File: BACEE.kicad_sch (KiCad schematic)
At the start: 13 parts, among them U1 24LC1025, U2 ATMEGA328-AU, U3 DS1337_PD, Y1 Crystal, Y2 Crystal

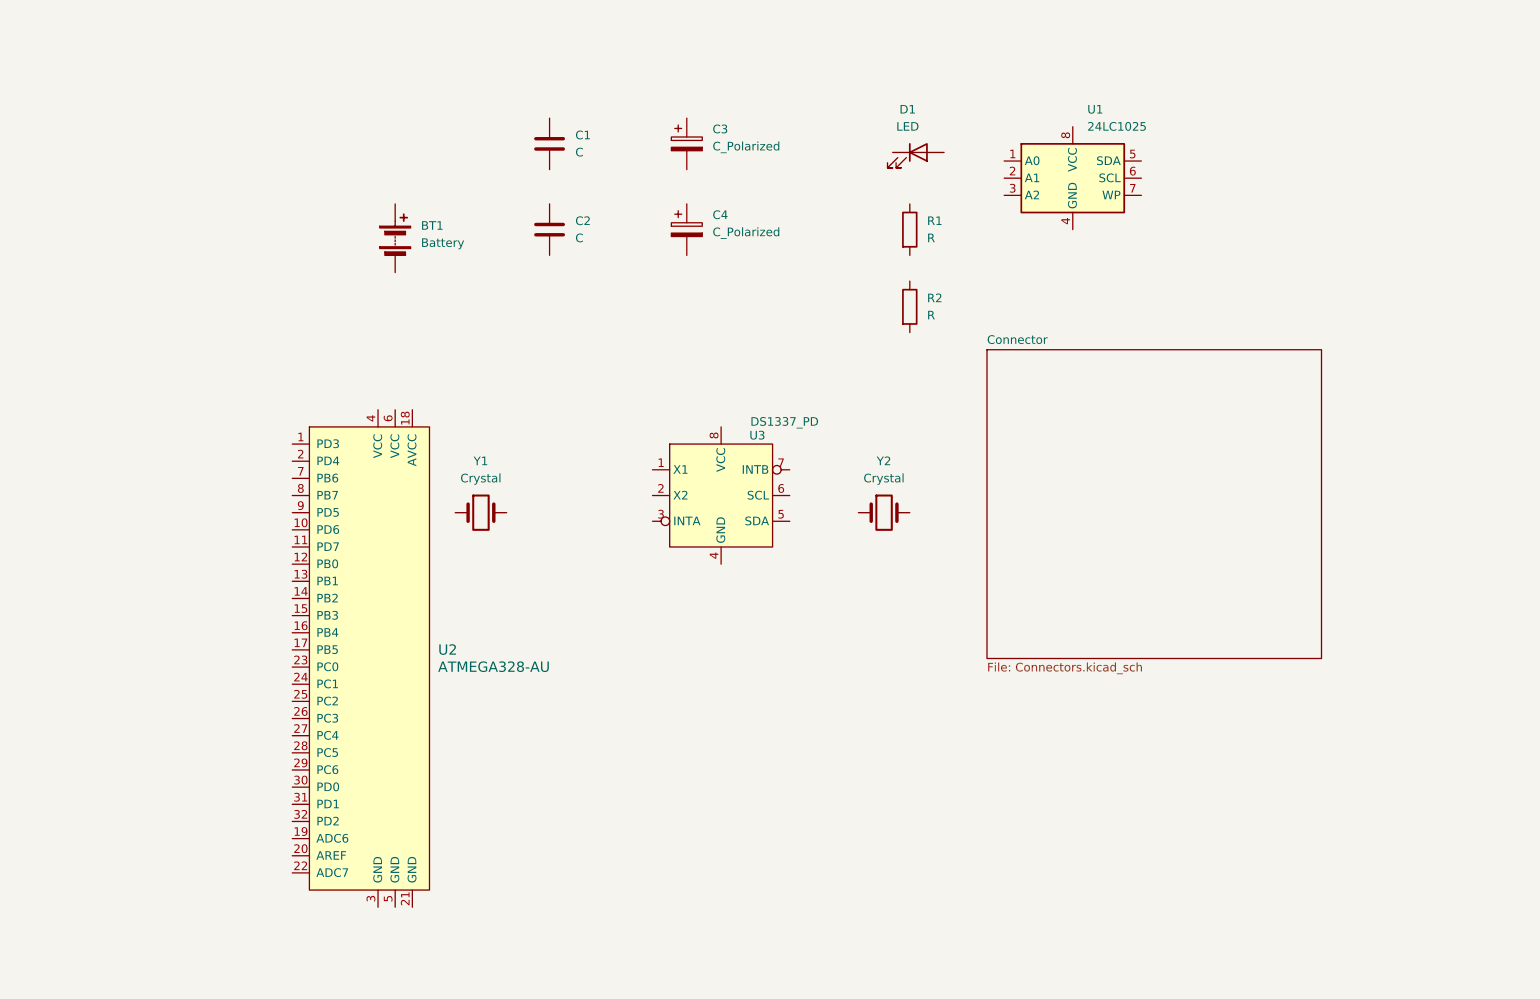
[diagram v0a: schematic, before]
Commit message: Arranged symbols
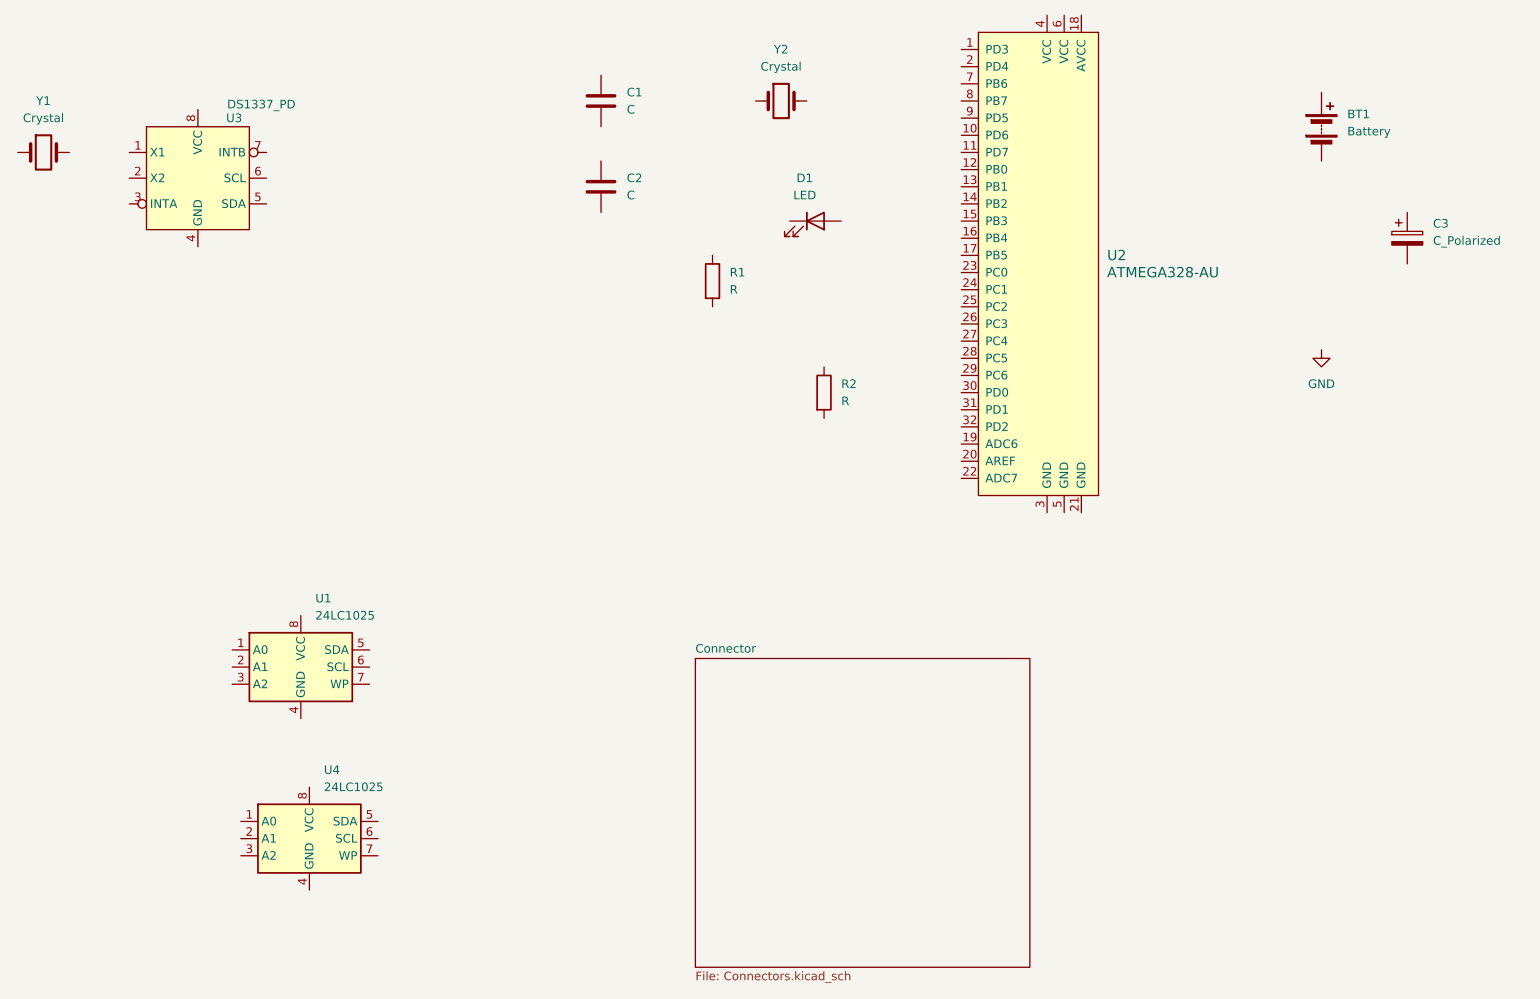
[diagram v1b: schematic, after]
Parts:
- removed C4: C_Polarized, symbol Device:C_Polarized
- added U4: 24LC1025, symbol Memory_EEPROM:24LC1025
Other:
- moved on the sheet: BT1, C1, C2, C3, D1, R1, R2, U1, U2, U3, Y1, Y2
